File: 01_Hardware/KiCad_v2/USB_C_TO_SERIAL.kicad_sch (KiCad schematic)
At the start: 25 parts, among them J100 TYPE-C-31-M-12, Q100 UMH3N, U100 USBLC6-2P6, U101 CP2102N-A02-GQFN24R

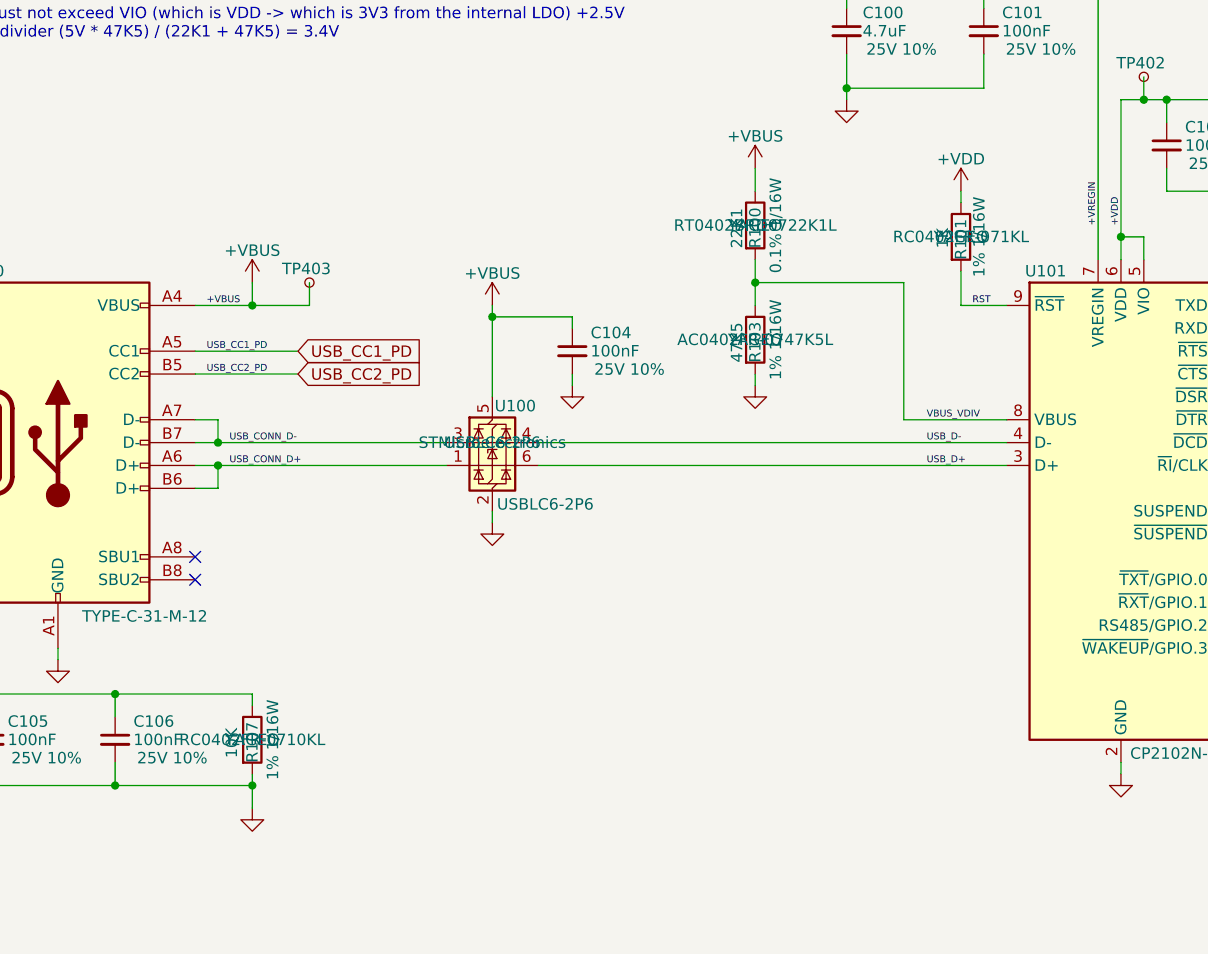
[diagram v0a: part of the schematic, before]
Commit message: USB-C and Serial PCB routing done
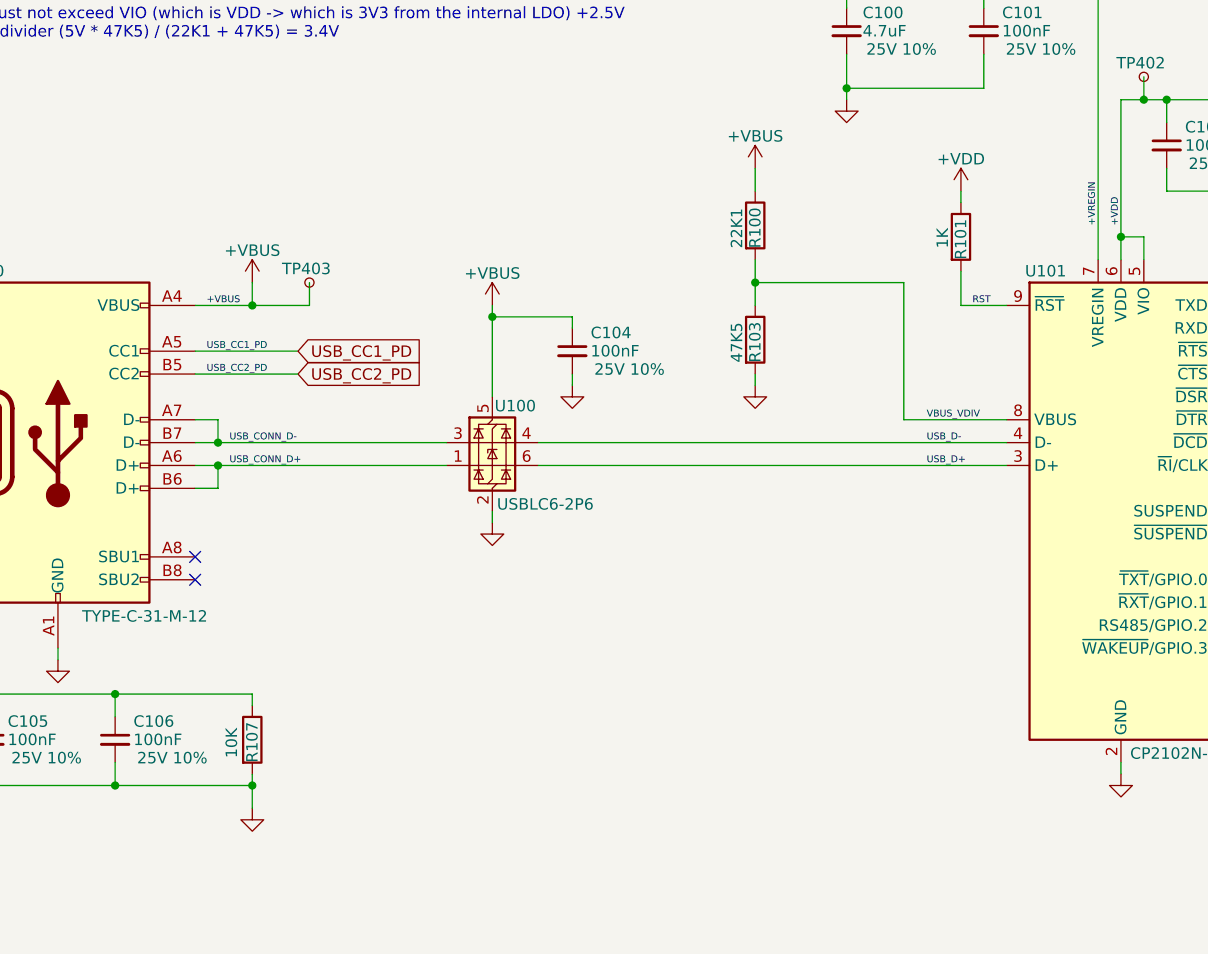
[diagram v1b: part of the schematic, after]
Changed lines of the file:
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@@
 					(size 1.27 1.27)
 				)
+				(hide yes)
 			)
 		)
@@
 					(size 1.27 1.27)
 				)
+				(hide yes)
 			)
 		)
@@
 					(size 1.27 1.27)
 				)
+				(hide yes)
 			)
 		)
@@
 					(size 1.27 1.27)
 				)
+				(hide yes)
 			)
 		)
@@
 					(size 1.27 1.27)
 				)
+				(hide yes)
 			)
 		)
@@
 					(size 1.27 1.27)
 				)
+				(hide yes)
 			)
 		)
@@
 					(size 1.27 1.27)
 				)
+				(hide yes)
 			)
 		)
@@
 					(size 1.27 1.27)
 				)
+				(hide yes)
 			)
 		)
@@
 					(size 1.27 1.27)
 				)
+				(hide yes)
 			)
 		)
@@
 					(size 1.27 1.27)
 				)
+				(hide yes)
 			)
 		)
@@
 					(size 1.27 1.27)
 				)
+				(hide yes)
 			)
 		)
@@
 					(size 1.27 1.27)
 				)
+				(hide yes)
 			)
 		)
@@
 					(size 1.27 1.27)
 				)
+				(hide yes)
 			)
 		)
@@
 					(size 1.27 1.27)
 				)
+				(hide yes)
 			)
 		)
@@
 					(size 1.27 1.27)
 				)
+				(hide yes)
 			)
 		)
@@
 					(size 1.27 1.27)
 				)
+				(hide yes)
 			)
 		)
@@
 					(size 1.27 1.27)
 				)
+				(hide yes)
 			)
 		)
@@
 					(size 1.27 1.27)
 				)
+				(hide yes)
 			)
 		)
@@
 					(size 1.27 1.27)
 				)
+				(hide yes)
 			)
 		)
@@
 					(size 1.27 1.27)
 				)
+				(hide yes)
 			)
 		)
@@
 					(size 1.27 1.27)
 				)
+				(hide yes)
 			)
 		)
@@
 					(size 1.27 1.27)
 				)
+				(hide yes)
 			)
 		)
@@
 					(size 1.27 1.27)
 				)
+				(hide yes)
 			)
 		)
@@
 					(size 1.27 1.27)
 				)
-			)
-		)
+				(hide yes)
+			)
+		)
